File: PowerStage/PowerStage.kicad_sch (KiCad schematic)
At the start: 27 parts, among them J1 Conn_01x02, J2 Conn_01x02, J3 Conn_01x03, Q1 IRFZ44N, Q2 IRFZ44N, SW2 SW_SPDT_XKB_DMx-xxxx-1, U1 IR2110

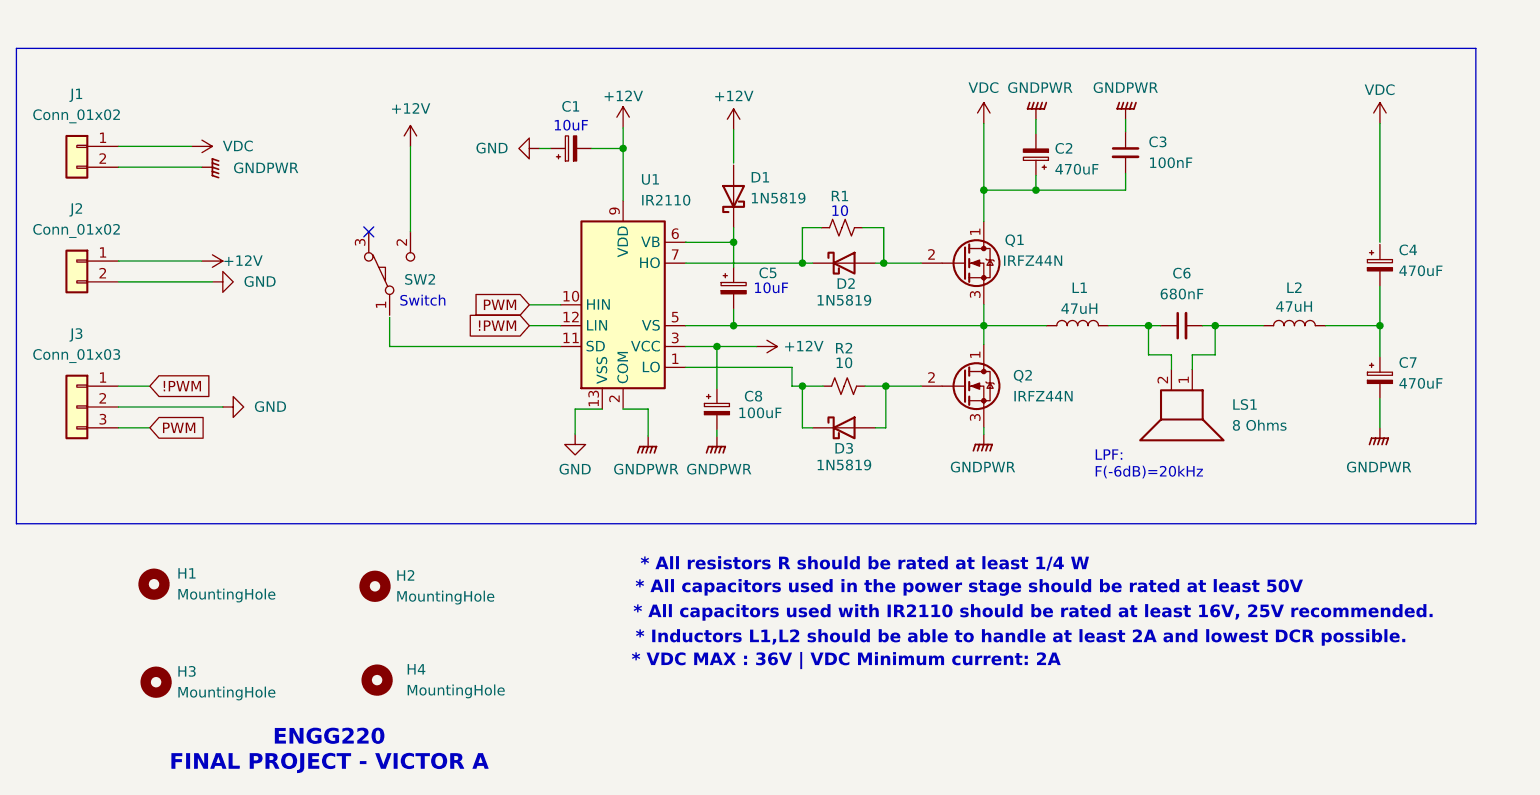
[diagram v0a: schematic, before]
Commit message: Created schematic pdf
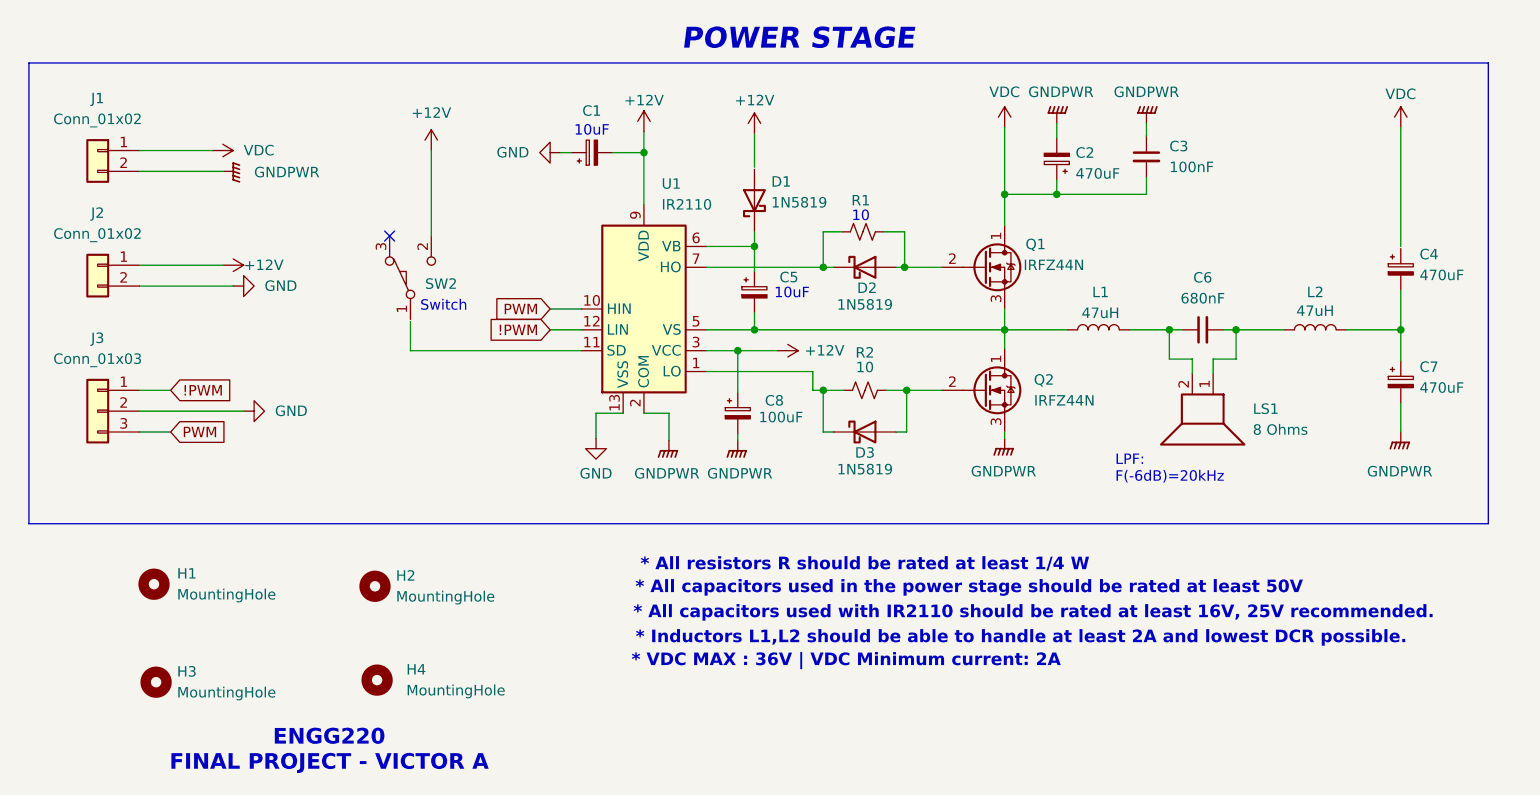
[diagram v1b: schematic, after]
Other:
- note added: "POWER STAGE"
- moved on the sheet: C1, C2, C3, C4, C5, C6, C7, C8, D1, D2, D3, J1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
